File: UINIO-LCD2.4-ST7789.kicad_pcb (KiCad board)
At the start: 2 copper layers, 69.3 x 48.7 mm, 37 parts, among them CON1 FFC_8Pin_0.5mm, J1 Conn_01x08_Male, Q1 S8050, U1 ME6211C33M5G-N, U2 AMS1117, U3 XC6206P332MR, U4 CON_10Pin

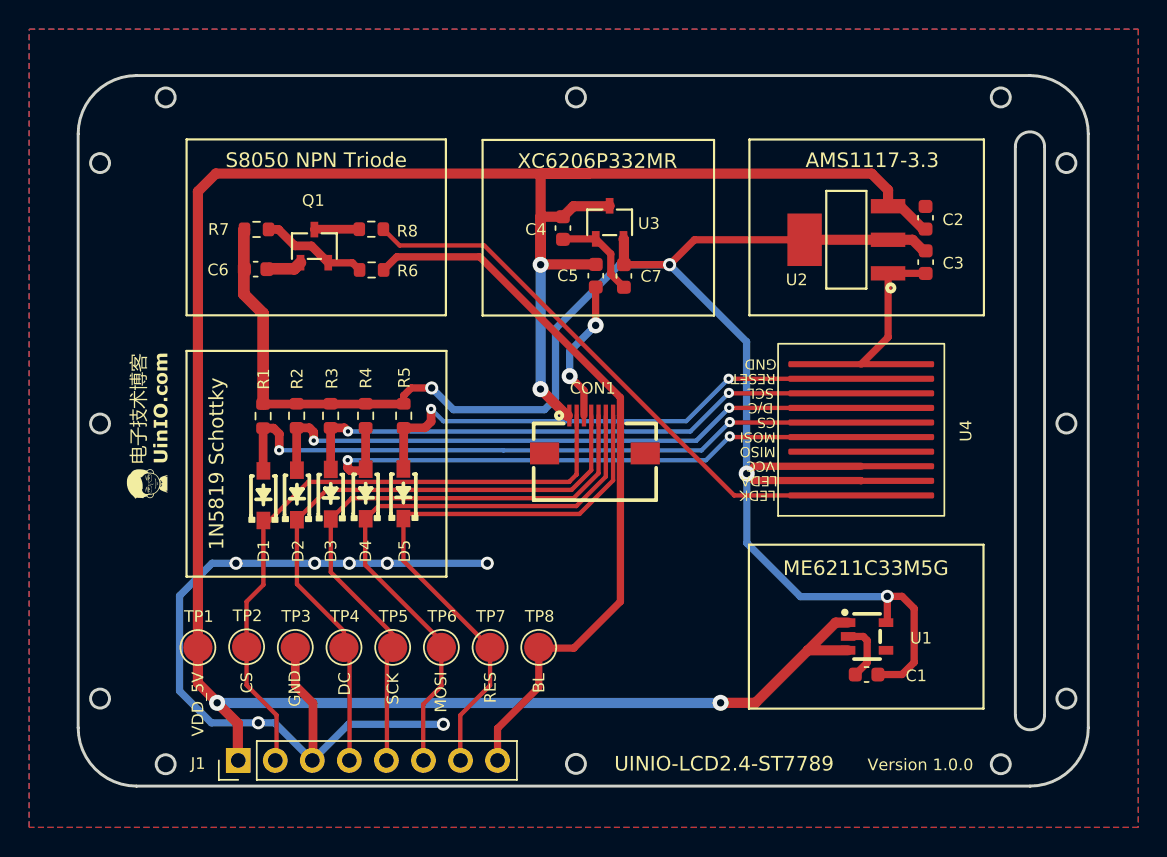
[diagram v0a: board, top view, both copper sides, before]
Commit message: Release UINIO-LCD2.4-ST7789
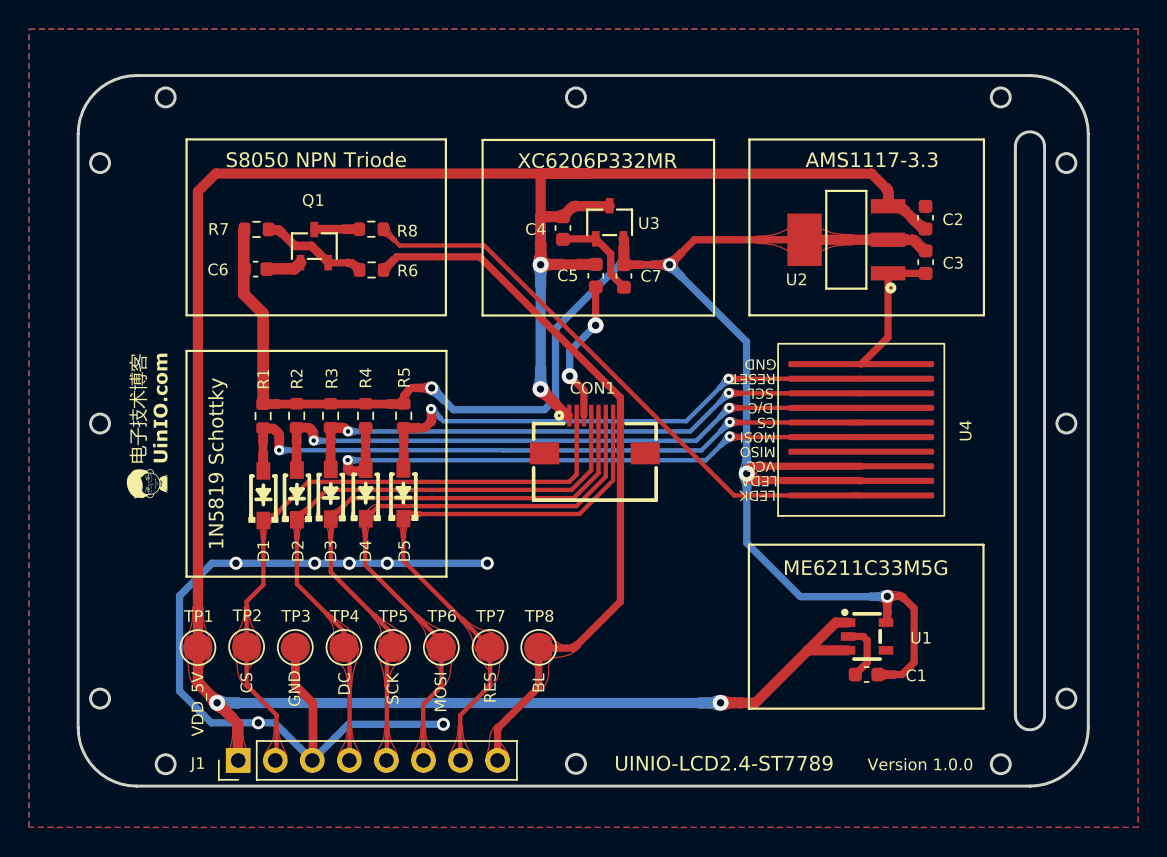
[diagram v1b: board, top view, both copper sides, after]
